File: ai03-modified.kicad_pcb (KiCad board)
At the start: 2 copper layers, 38.1 x 45.2 mm, 20 parts, among them SW1 SW_Push, U1 ATmega32U4-A, Y1 16MHz

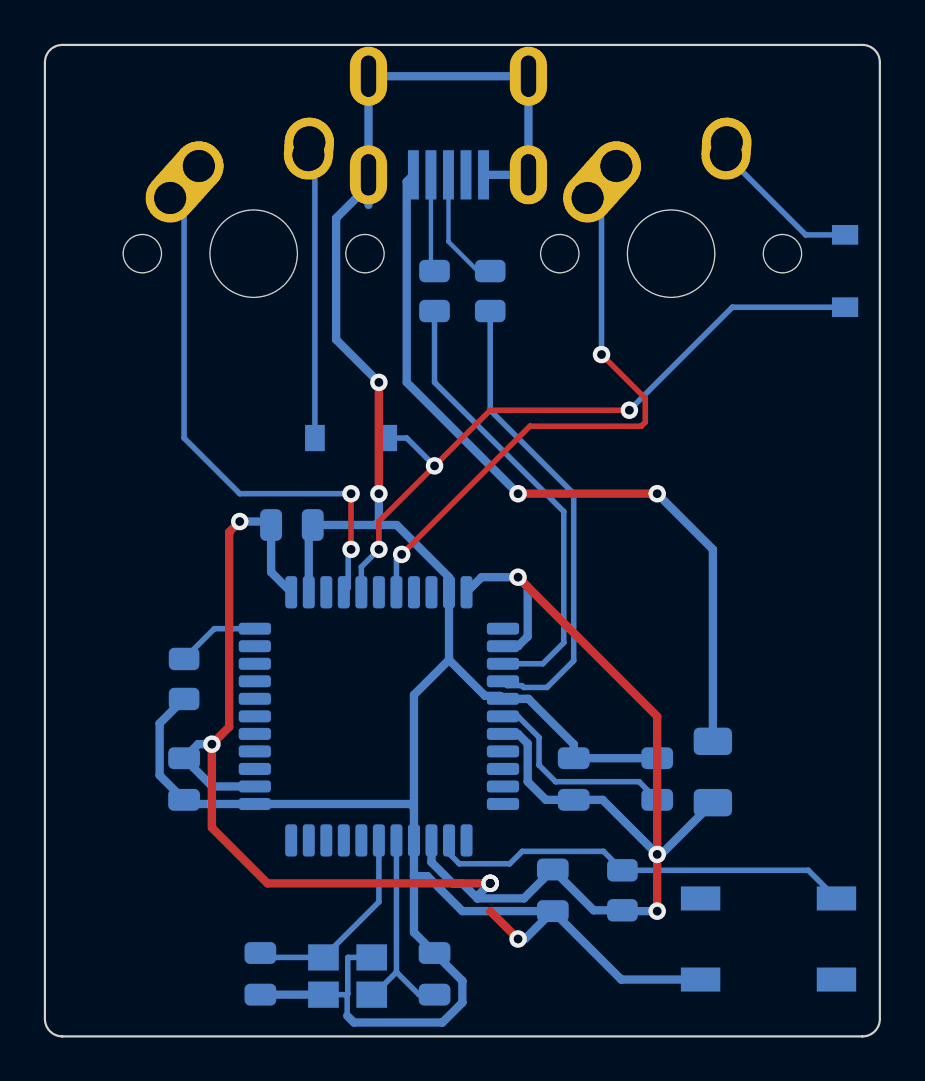
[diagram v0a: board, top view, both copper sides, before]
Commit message: FillZone
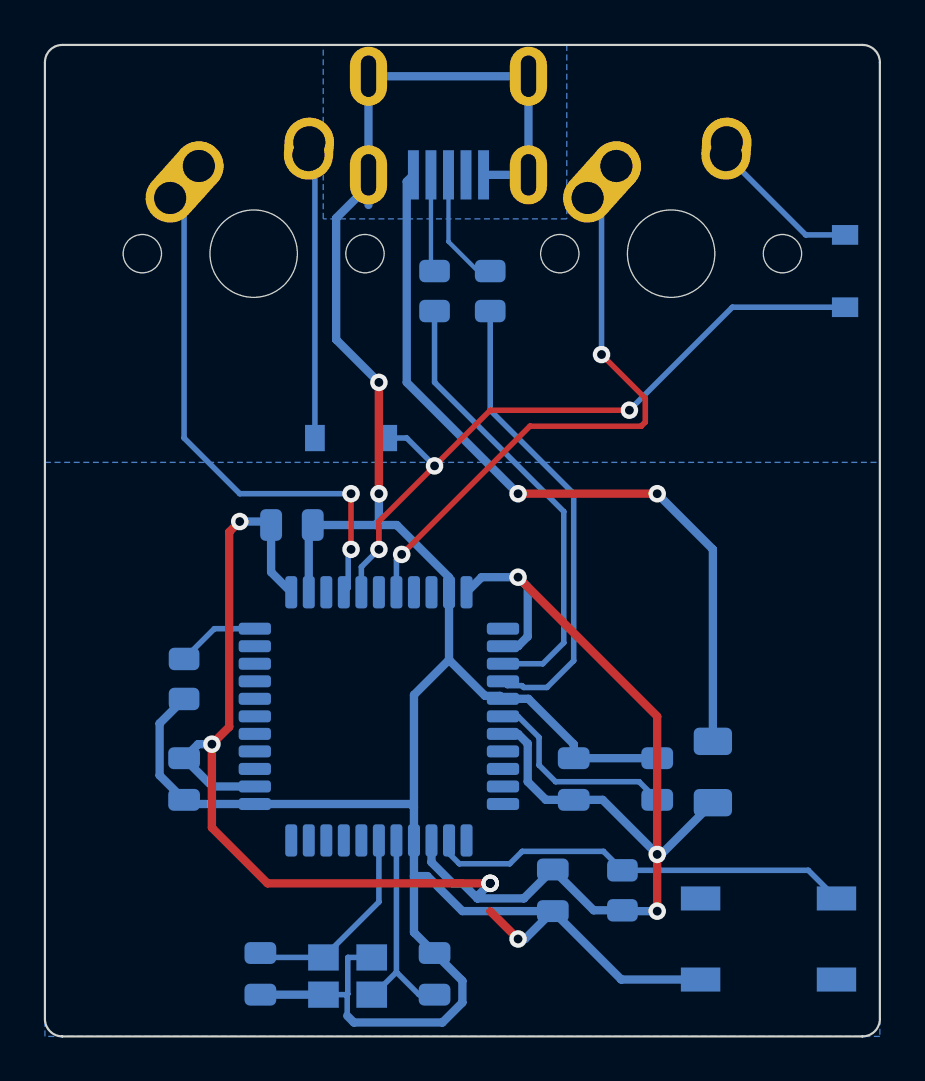
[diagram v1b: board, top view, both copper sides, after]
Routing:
- added copper zone on B.Cu, net GND
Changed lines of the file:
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@@
   (segment (start 88.9 111.76) (end 88.9 105.25125) (width 0.254) (layer "B.Cu") (net 41))
   (segment (start 79.972425 120.687575) (end 79.779737 120.880262) (width 0.254) (layer "B.Cu") (net 41))
+  (zone (net 2) (net_name "GND") (layer "B.Cu") (hatch edge 0.508)
+    (connect_pads (clearance 0.508))
+    (min_thickness 0.254) (filled_areas_thickness no)
+    (fill yes (thermal_gap 0.508) (thermal_bridge_width 0.508))
+    (polygon
+      (pts
+        (xy 87.3125 105.56875)
+        (xy 76.2 105.56875)
+        (xy 76.2 97.63125)
+        (xy 87.3125 97.63125)
+      )
+    )
+  )
+  (zone (net 2) (net_name "GND") (layer "B.Cu") (hatch edge 0.508)
+    (connect_pads (clearance 0.508))
+    (min_thickness 0.254) (filled_areas_thickness no)
+    (fill yes (thermal_gap 0.508) (thermal_bridge_width 0.508))
+    (polygon
+      (pts
+        (xy 101.6 142.875)
+        (xy 63.5 142.875)
+        (xy 63.5 116.68125)
+        (xy 101.6 116.68125)
+      )
+    )
+  )
 )
